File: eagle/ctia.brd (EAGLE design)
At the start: 96.8 x 97.7 mm, 16 parts, among them IC1 IVC102UADAPTOR, IC2 LT1352PA, IC3 AD580H

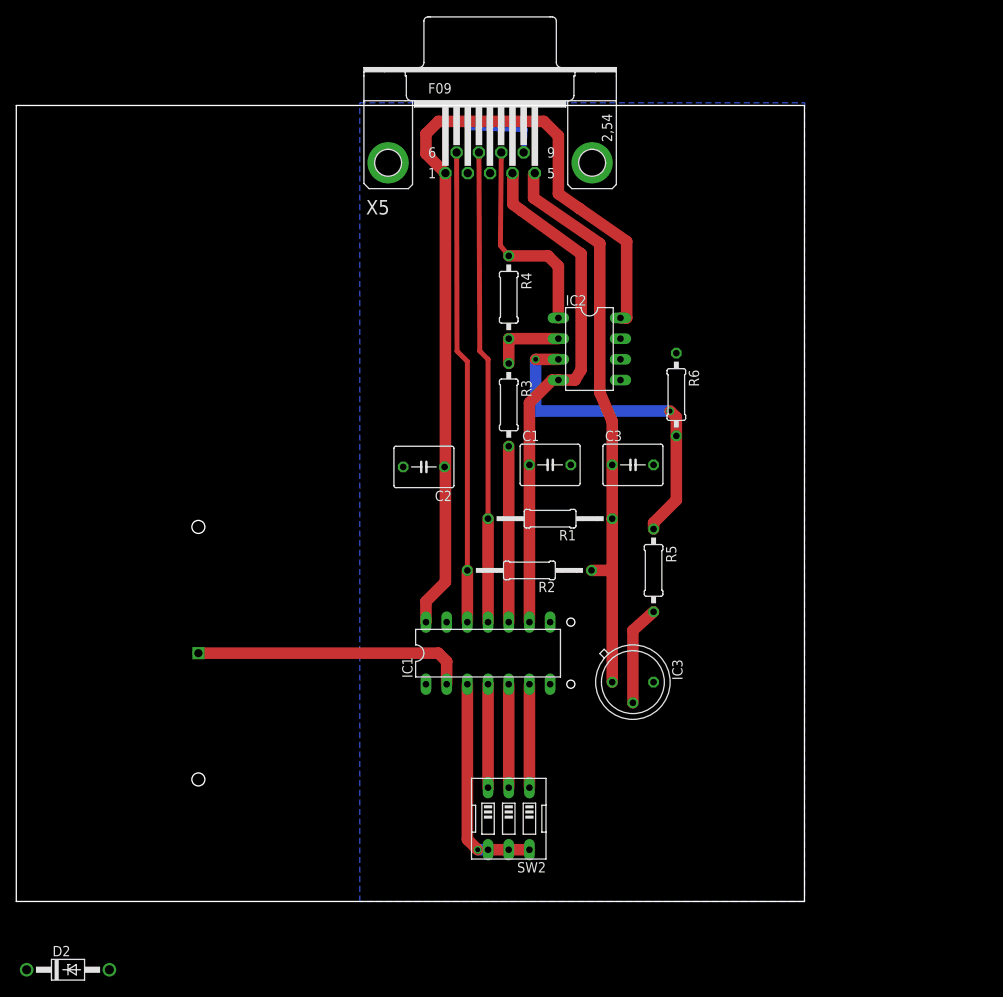
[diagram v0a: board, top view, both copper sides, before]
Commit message: lower noise
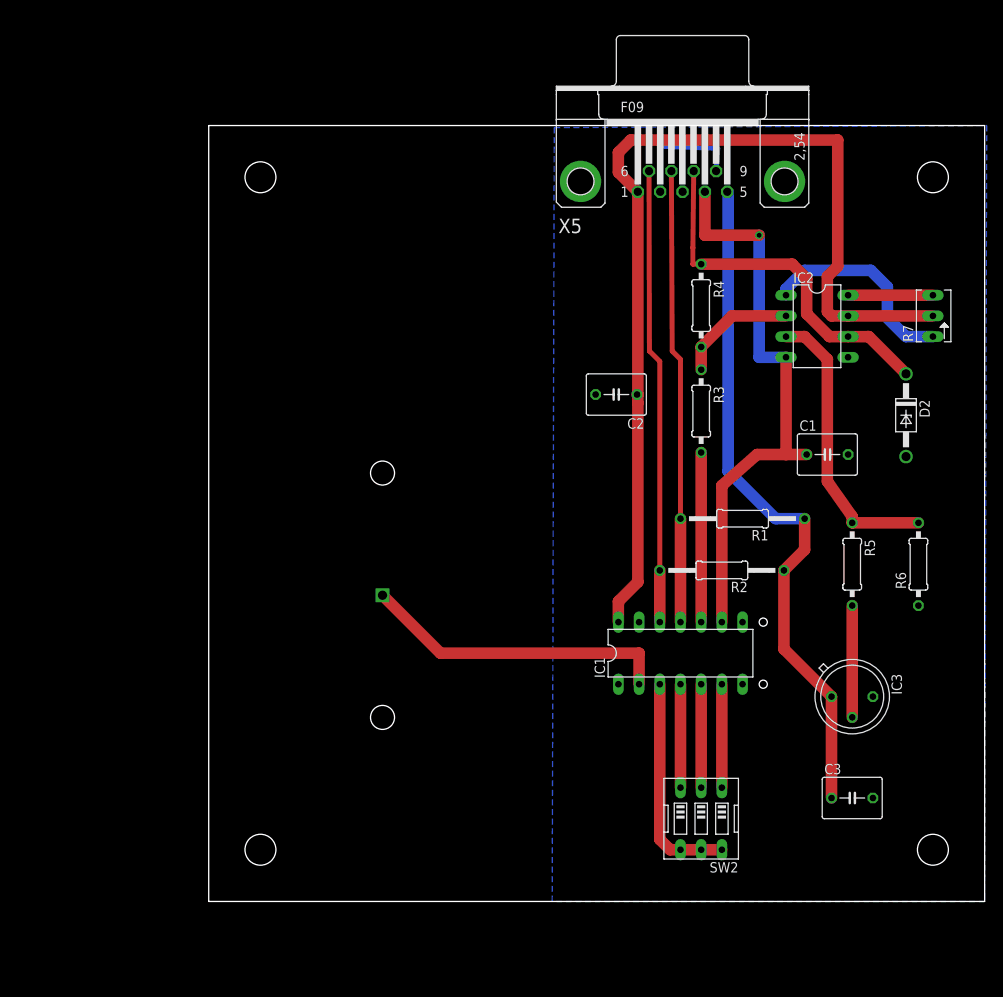
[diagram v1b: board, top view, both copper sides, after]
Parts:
- added R7: 10k, pot:B64Y
- IC2: value LT1352PA -> OPA27GP; device linear-technology:DIL08 -> linear:DIL08
- R3, R6: value 10k -> 1M
- R4, R5: value 1.5M -> 1M
- moved D2 123.4 mm to (85.6, 59.7), turned to 270 degrees
- moved C3 49.0 mm to (79.0, 12.7)
- moved R6 36.3 mm to (87.1, 41.4), turned to 90 degrees
- moved C1 34.1 mm to (75.9, 54.9)
- moved IC2 28.1 mm to (74.7, 70.6)
- moved IC3 27.0 mm to (79.0, 25.1)
- moved C2 25.2 mm to (50.0, 62.2)
- moved R5 24.4 mm to (79.0, 41.4)
- moved X5 23.7 mm to (58.2, 88.4)
- moved U$1 23.7 mm to (21.3, 37.6)
- moved R4 23.6 mm to (60.5, 73.2)
- moved R3 23.6 mm to (60.5, 60.2)
- moved IC1 23.6 mm to (57.9, 30.5)
- moved R1 23.6 mm to (65.5, 47.0)
- moved R2 23.6 mm to (63.0, 40.6)
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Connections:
- new net N$10: IC2.8, R7.A
- new net N$9: IC2.1, R7.E
- net +15V: now also IC2.7, R7.S; no longer IC2.8
- net VOUT: now also IC2.6; no longer IC2.1
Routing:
- net N$9: track 0.00 -> 25.3 mm
- net VOUT: track 26.0 -> 45.7 mm
- net +15V: track 107.0 -> 122.1 mm
- net +5V: track 69.7 -> 83.9 mm
- net N$10: track 0.00 -> 10.4 mm
- net -15V: track 63.6 -> 70.8 mm
- net N$7: track 41.6 -> 35.4 mm, vias 2 -> 0
- net N$6: track 9.14 -> 14.8 mm
- net VIN: track 33.7 -> 38.3 mm
- net RESET: track 58.2 -> 55.9 mm
- net SAMPLE: track 58.1 -> 55.8 mm
- net N$8: track 12.3 -> 13.7 mm
- net N$5: track 21.6 -> 20.8 mm
- net N$4: vias 1 -> 0
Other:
- board size 96.8 x 97.7 mm -> 95.2 x 95.2 mm
